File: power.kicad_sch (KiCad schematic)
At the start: 37 parts, among them J4 USB_C_Receptacle_USB2.0_16P, U2 BQ25170DSGR, U3 LM66100DCK, U5 TPS628438DRL, U6 LM66100DCK

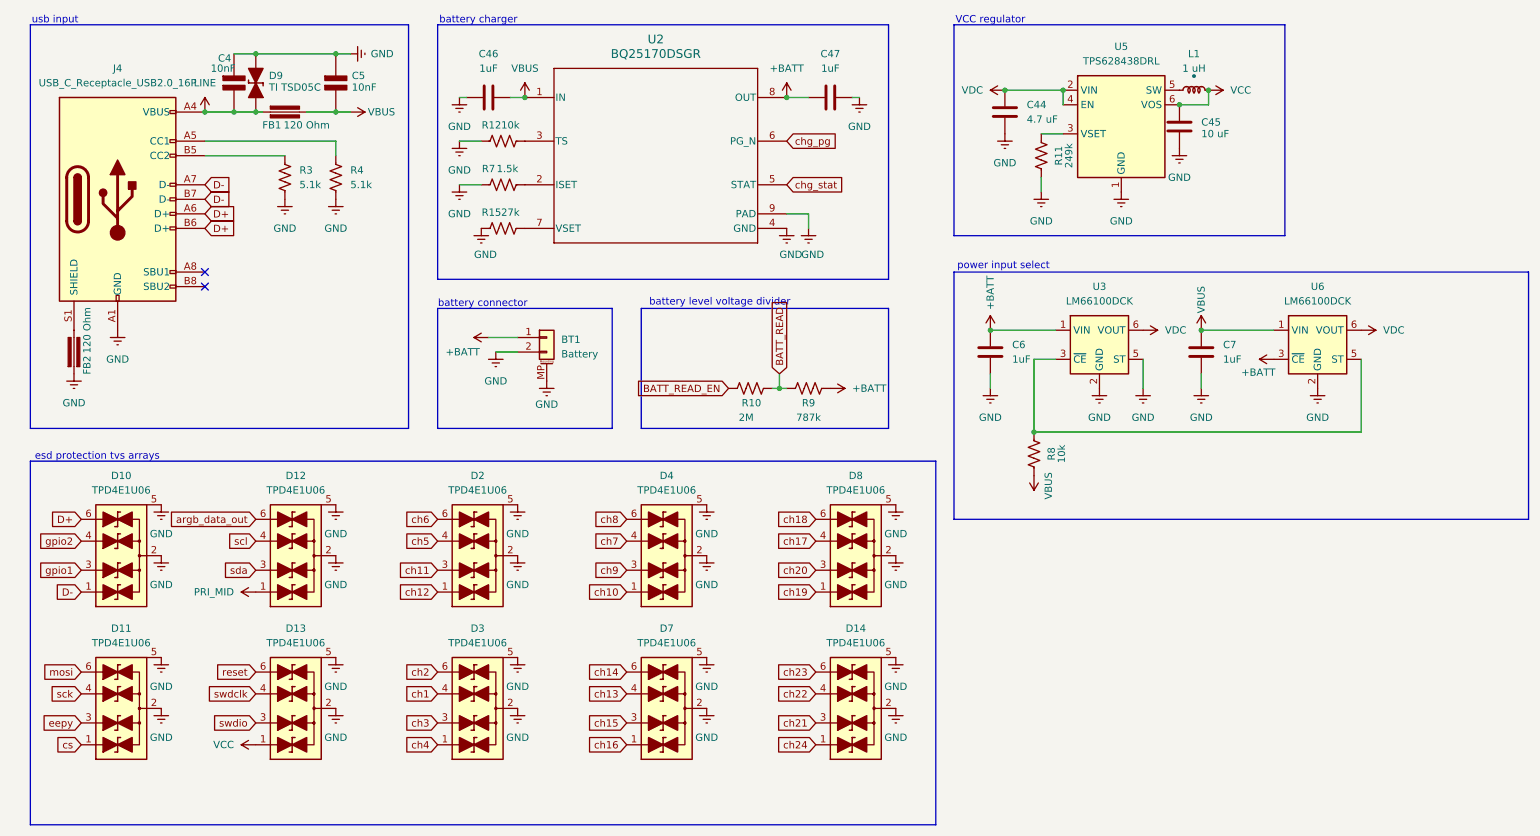
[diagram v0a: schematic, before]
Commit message: cleanup
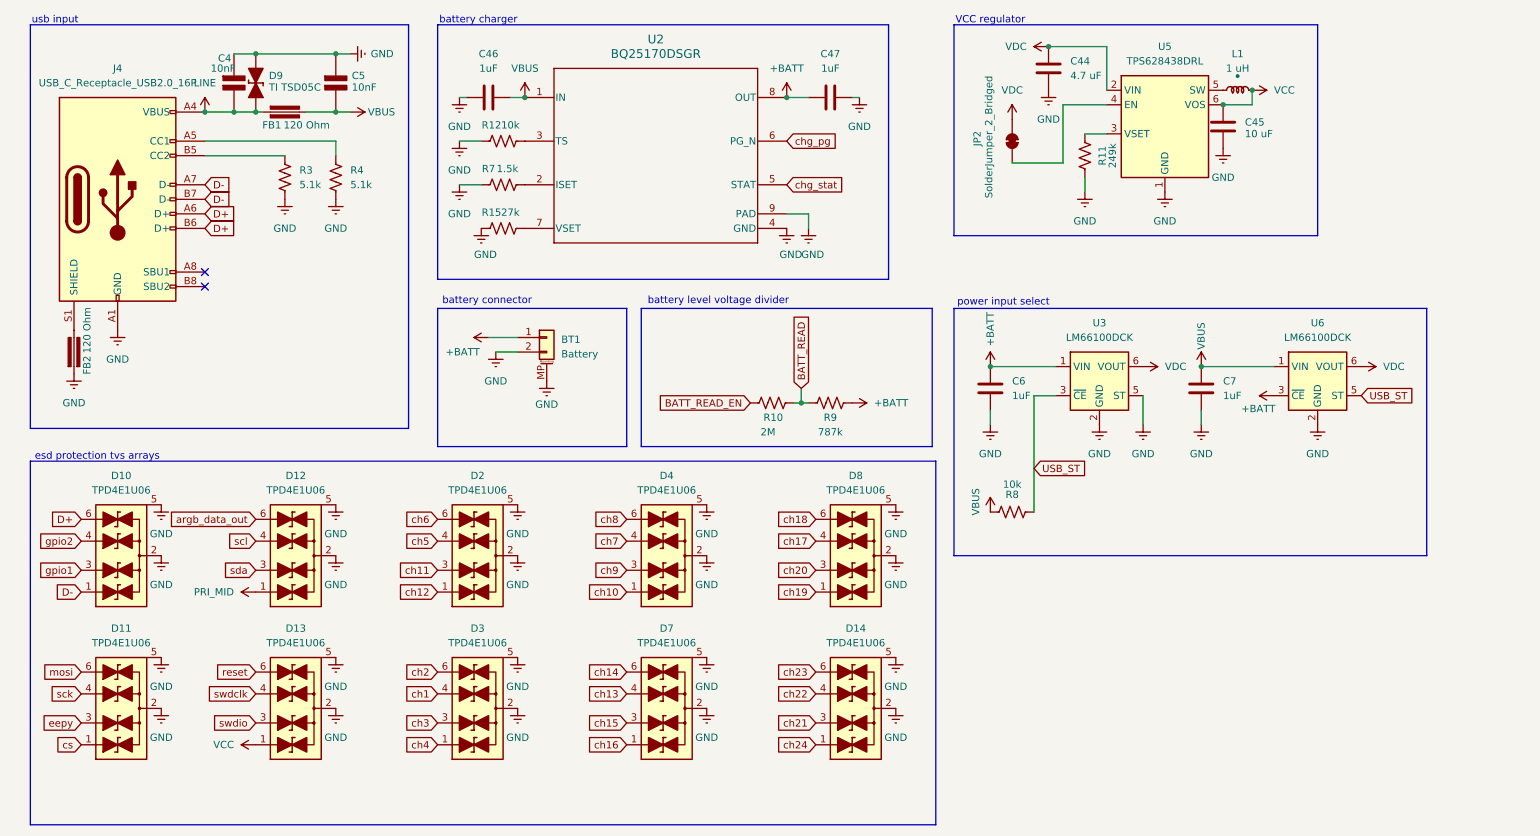
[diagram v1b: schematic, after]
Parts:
- added JP2: SolderJumper_2_Bridged, Jumper:SolderJumper-2_P1.3mm_Bridged_RoundedPad1.0x1.5mm, symbol Jumper:SolderJumper_2_Bridged
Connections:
- net VBUS: now also R8.1; no longer R8.2
- net VDC: now also JP2.1 (A); no longer U5.4 (EN)
- net USB_ST: now reaches U3.3 (~{CE}), U6.5 (ST)
- net USB_ST: now also R8.2; no longer R8.1
- new net: JP2.2 (B), U5.4 (EN)
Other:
- moved on the sheet: C44, C45, C6, C7, L1, R10, R11, R8, R9, U3, U5, U6
